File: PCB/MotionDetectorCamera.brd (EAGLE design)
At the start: 41.9 x 32.6 mm, 185 parts, among them J1 JUMPER-SOLDER, J10 MICROSD-SOCKET, J11 USB-C-JACK, J2 JUMPER-SOLDER, J3 JUMPER-SOLDER, J4 JUMPER-SOLDER, J5 JST-SM02B-SRSS-TB, J6 JUMPER-SOLDER, J7 JUMPER-SOLDER, J8 JUMPER-SOLDER, J9 S-MOUNT-LENS-HOLDERM12LENSES-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, Q1 PMOS-NEXPERIA-SOT1220, Q2 PMOS-NEXPERIA-SOT1220, Q3 PMOS-NEXPERIA-SOT1220, U1 TI-TPS2116, U10 TI-TPS22919DCK, U11 TI-TPS62A01, U13 TI-TPS22919DCK, U14 TI-TPS22919DCK, U15 TI-MSP430FR2422IRHL, U16 NXP-NTB0102, U17 NXP-NTB0102, U18 PANASONIC-EKMB110711X, U19 LATTICE-ICE40HX4K-BG121, U2 DIODESINC-AP7350, U20 WINBOND-W25Q40EW, U21 NEXPERIA-74LVC1G98-OR-INV-INP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, U22 NEXPERIA-74LVC1G98-BUFFER, U23 ON-AR0330CS1C12SPKA0, U24 ALLIANCE-AS4C8M16MSA-6BIN, U25 STM-STM32F730, U26 DIODESINC-DT1446-04V-7, U27 NEXPERIA-74LVC1G98-BUFFER, U3 NEXPERIA-74LVC1G98-NOR, U4 MICROCHIP-MCP7383X, U5 EATON-STN101, U6 TI-TPS62A01, U7 TI-TPS62A01, U9 TI-TPS22919DCK, X1 EPSON-FC-135, X2 SITIME-SIT8021, X3 SITIME-SIT8021

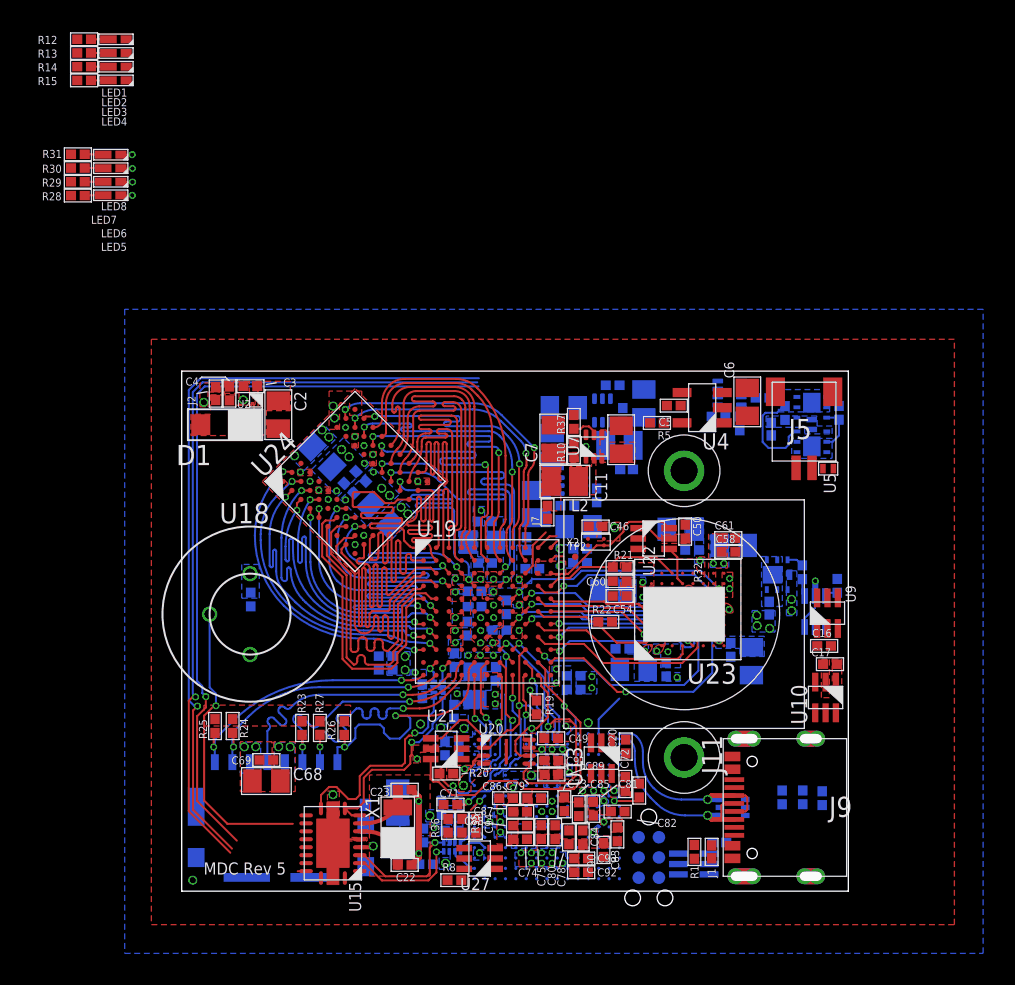
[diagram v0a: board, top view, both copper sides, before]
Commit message: Layout progress
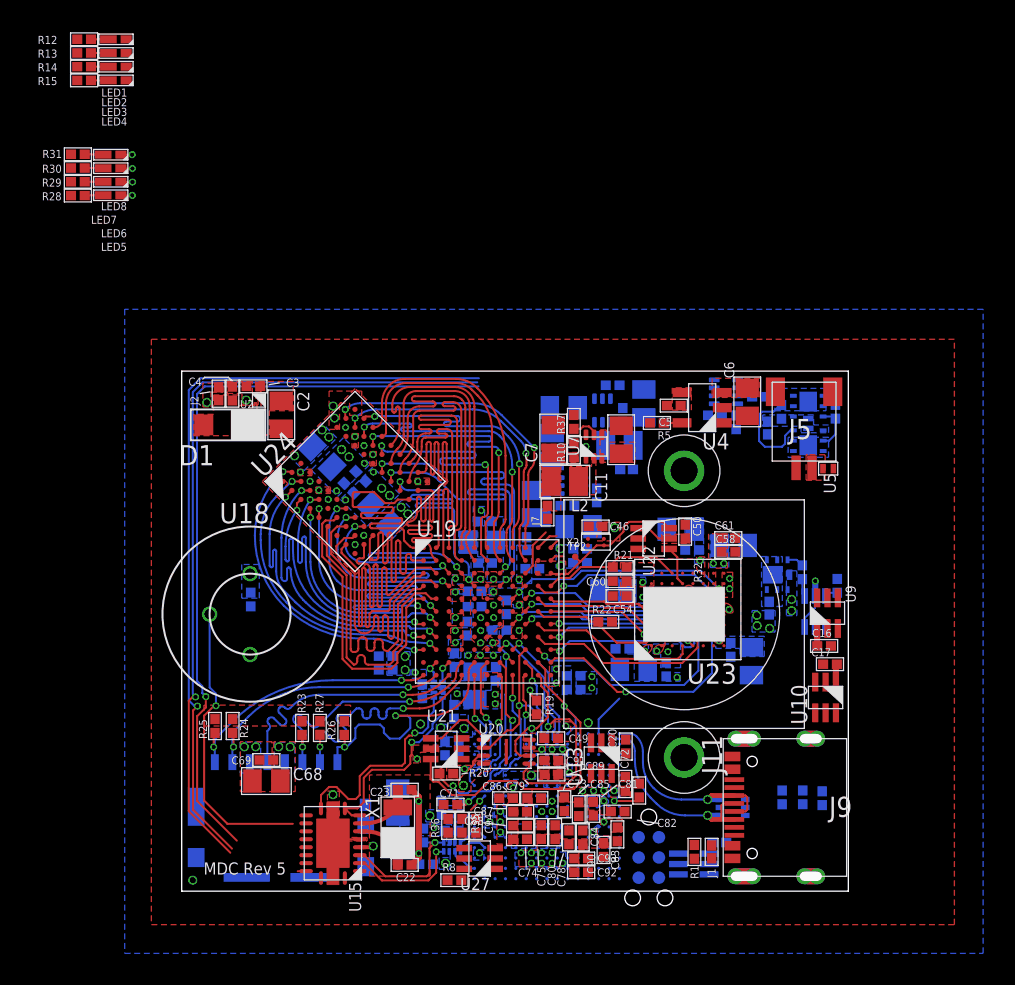
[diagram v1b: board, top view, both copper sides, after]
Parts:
- moved C1 0.23 mm to (36.2, 31.0)
- moved J4 0.23 mm to (36.8, 29.1)
- moved Q3 0.23 mm to (39.3, 28.3)
- moved R2 0.23 mm to (33.5, 29.9)
- moved R7 0.23 mm to (37.7, 30.1)
- moved R9 0.23 mm to (41.0, 30.1)
- moved U1 0.23 mm to (34.2, 31.3)
- moved Q2 0.23 mm to (39.3, 30.4)
- moved R3 0.23 mm to (34.8, 29.4)
- moved C2 0.19 mm to (6.25, 29.9)
- moved C3 0.19 mm to (4.50, 31.7)
- moved C4 0.19 mm to (3.18, 31.2)
- moved D1 0.19 mm to (2.91, 29.3)
- moved J2 0.19 mm to (2.32, 31.2)
- moved U2 0.19 mm to (4.85, 30.8)
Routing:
- net VDD_A_3V3: track 95.1 -> 84.2 mm
- net VDD_B_3V3_STM: track 7.24 -> 0.64 mm
- net VDD_B_2V8: track 60.8 -> 61.9 mm
- net N$21: track 0.00 -> 1.15 mm
- net VDD_B_1V8: track 3.54 -> 4.63 mm
- added copper zone on layer 1, net VDD_BAT
- added copper zone on layer 1, net VDD_BAT_IN
- added copper zone on layer 1, net VDD_USB
